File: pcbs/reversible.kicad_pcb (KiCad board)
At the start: 2 copper layers, 132.7 x 86.8 mm, 50 parts

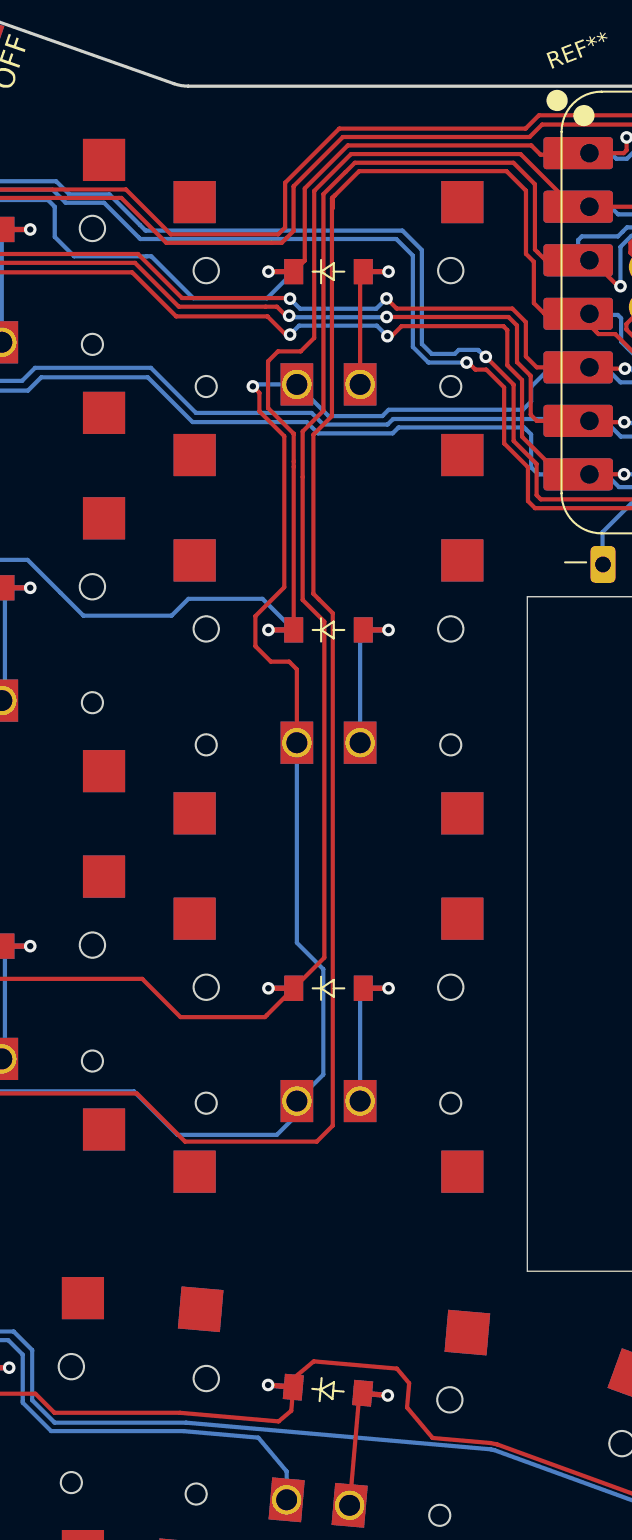
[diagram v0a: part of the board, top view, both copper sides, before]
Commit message: minor changes to the routing
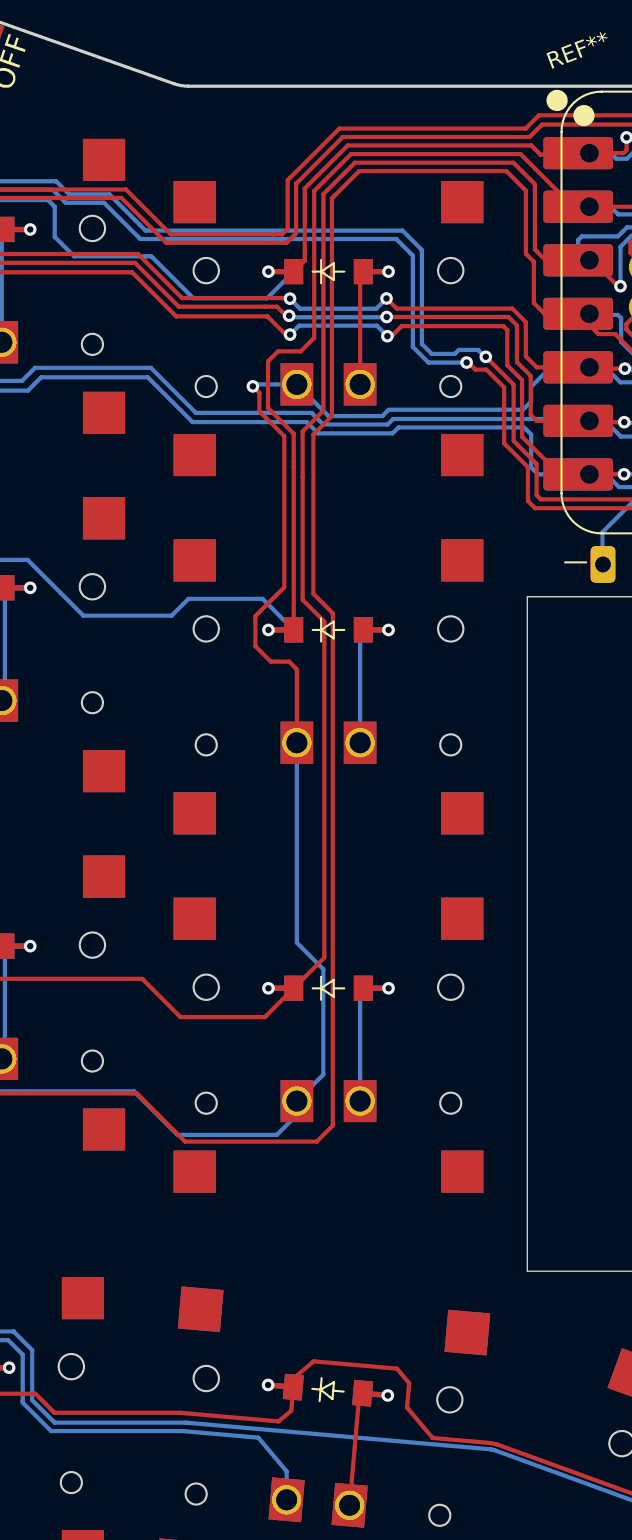
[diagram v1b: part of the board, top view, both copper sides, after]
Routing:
- net P3: track 168.2 -> 167.2 mm
